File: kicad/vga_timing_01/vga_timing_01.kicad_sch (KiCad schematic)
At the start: 13 parts, among them J1 DIN41612_02x32_AC, J2 UART1, J3 UART2, U10 TL28L92FR, U13 74AHC1G32, Y1 Crystal 3.6864MHz

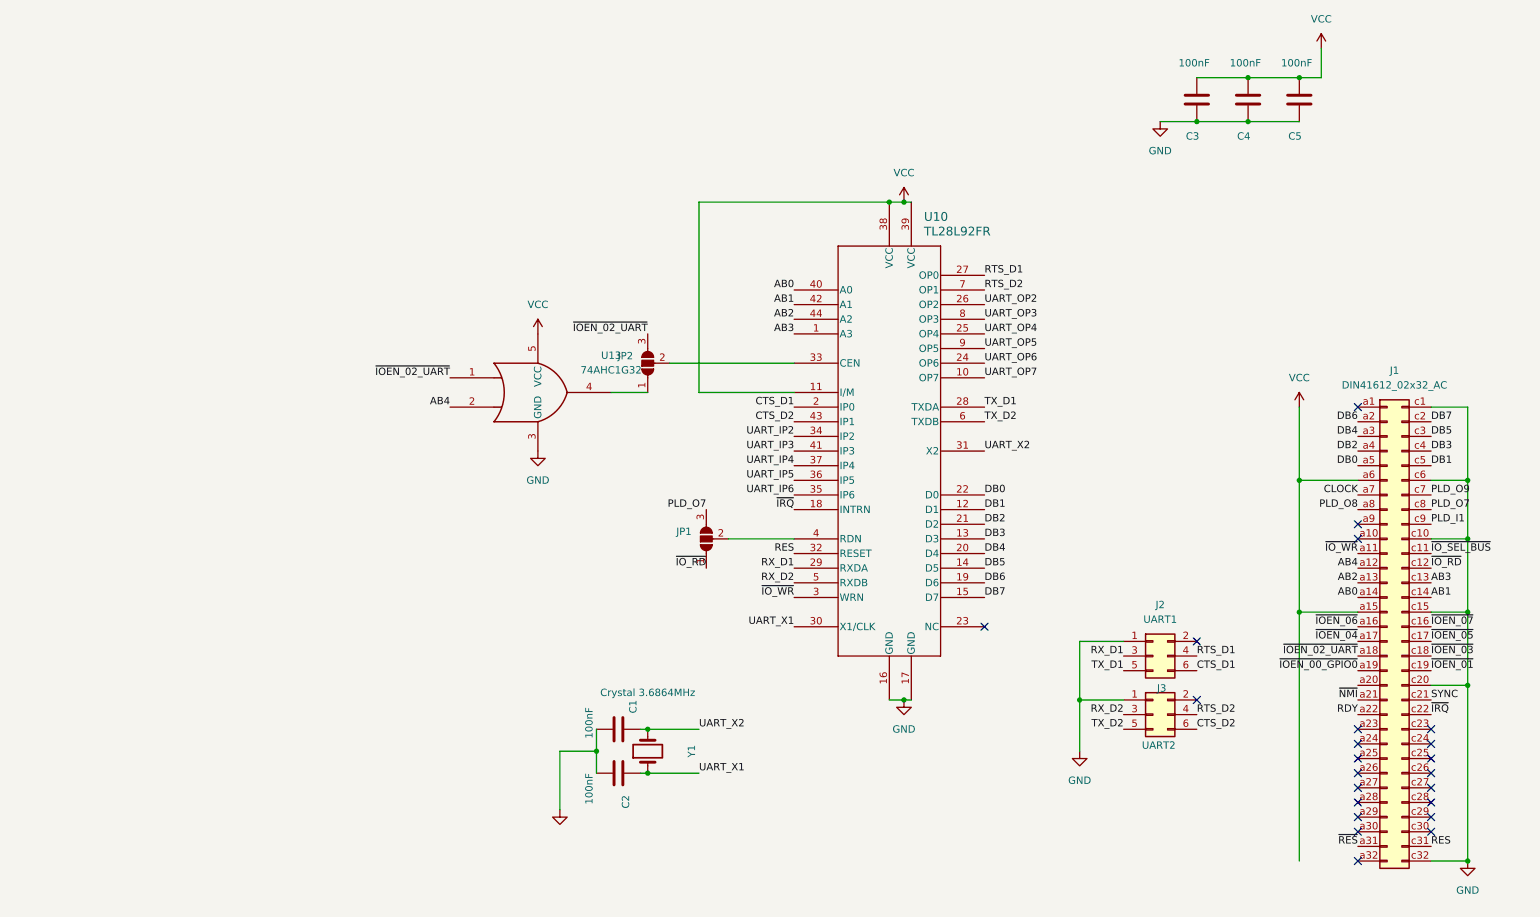
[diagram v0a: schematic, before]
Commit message: vga timing board 01 work
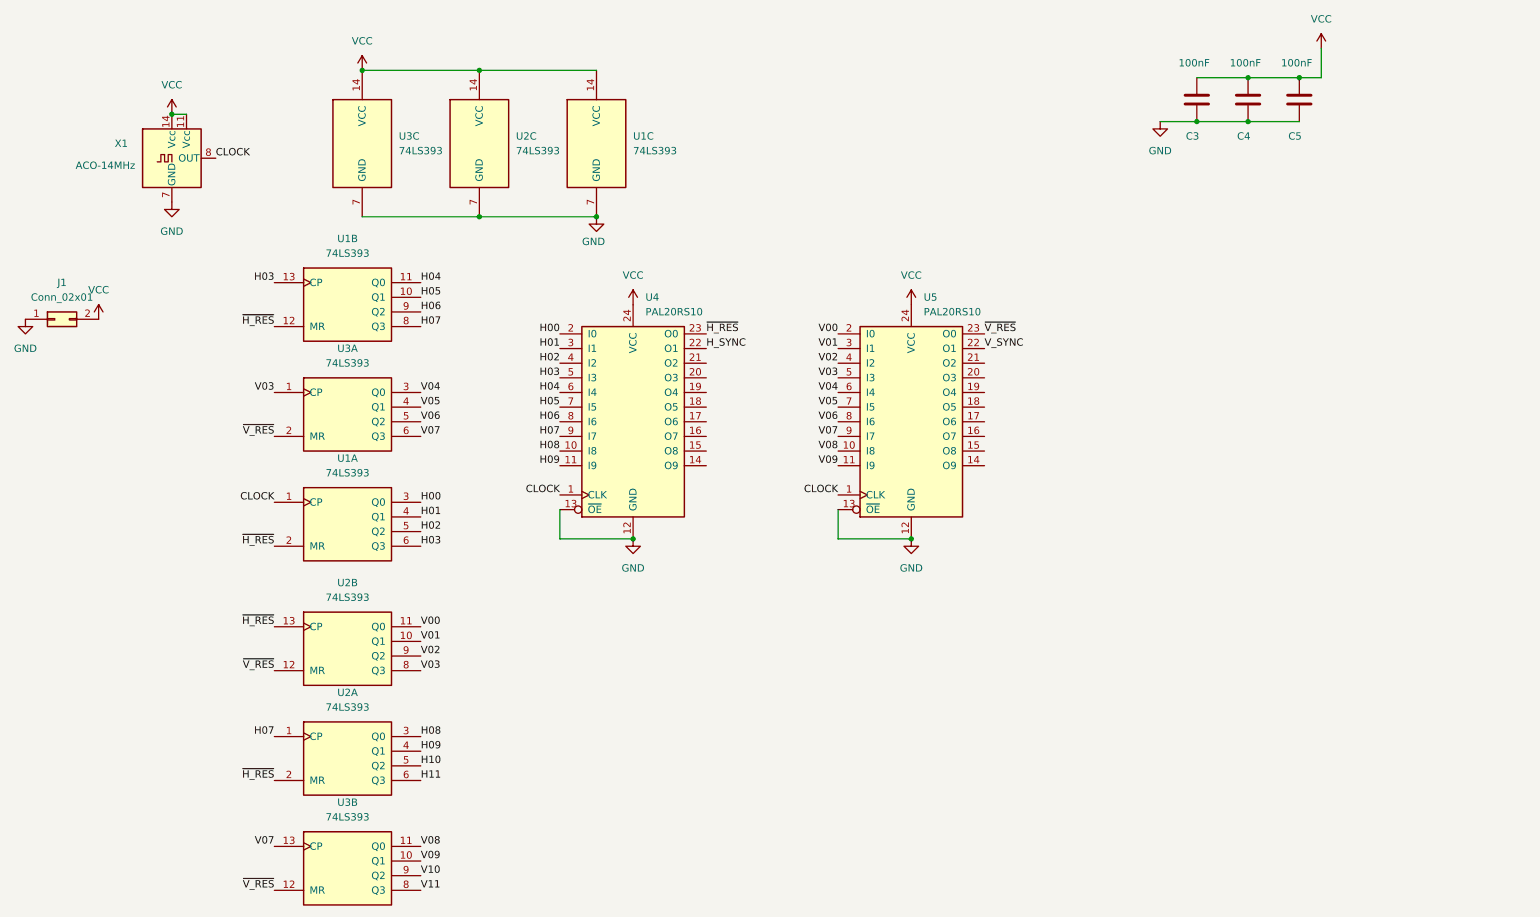
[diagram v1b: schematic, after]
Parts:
- removed C1, C2: 100nF, Capacitor_THT:C_Disc_D4.7mm_W2.5mm_P5.00mm, symbol Device:C
- removed J1: DIN41612_02x32_AC, Connector_DIN:DIN41612_C_2x32_Male_Horizontal_THT, symbol Connector:DIN41612_02x32_AC
- removed J2: UART1, Connector_PinHeader_2.54mm:PinHeader_2x03_P2.54mm_Horizontal, symbol Connector_Generic:Conn_02x03_Odd_Even
- removed J3: UART2, Connector_PinHeader_2.54mm:PinHeader_2x03_P2.54mm_Horizontal, symbol Connector_Generic:Conn_02x03_Odd_Even
- removed JP1, JP2: SolderJumper_3_Open, Jumper:SolderJumper-3_P1.3mm_Open_RoundedPad1.0x1.5mm_NumberLabels, symbol Jumper:SolderJumper_3_Open
- removed U10: TL28L92FR, Package_QFP:MQFP-44_10x10mm_P0.8mm, symbol 2024-09-25_17-04-06:TL28L92FR
- removed U13: 74AHC1G32, Package_TO_SOT_SMD:SOT-23-5_HandSoldering, symbol 74xGxx:74AHC1G32
- removed Y1: Crystal 3.6864MHz, Crystal:Crystal_HC49-4H_Vertical, symbol Device:Crystal
- added J1: Conn_02x01, Connector_PinSocket_1.27mm:PinSocket_2x01_P1.27mm_Vertical, symbol Connector_Generic:Conn_02x01
- added U1, U2, U3: 74LS393, Package_SO:SOIC-14_3.9x8.7mm_P1.27mm, symbol 74xx:74LS393
- added U4, U5: PAL20RS10, Package_DIP:DIP-24_W7.62mm_Socket, symbol Logic_Programmable:PAL20RS10
- added X1: ACO-14MHz, Package_DIP:DIP-14_W7.62mm_Socket, symbol 65xx:osci-14or8
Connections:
- net CLOCK: now also U1.1 (CP), U4.1 (CLK), U5.1 (CLK), X1.8 (OUT)
- net GND: now also J1.1 (Pin_1), U1.7 (GND), U2.7 (GND), U3.7 (GND), U4.12 (GND), U4.13 (~{OE}), U5.12 (GND), U5.13 (~{OE}), X1.7 (GND)
- net VCC: now also J1.2 (Pin_2), U1.14 (VCC), U2.14 (VCC), U3.14 (VCC), U4.24 (VCC), U5.24 (VCC), X1.11 (Vcc), X1.14 (Vcc)
- new net H00: U1.3 (Q0), U4.2 (I0)
- new net H01: U1.4 (Q1), U4.3 (I1)
- new net H02: U1.5 (Q2), U4.4 (I2)
- new net H03: U1.13 (CP), U1.6 (Q3), U4.5 (I3)
- new net H04: U1.11 (Q0), U4.6 (I4)
- new net H05: U1.10 (Q1), U4.7 (I5)
- new net H06: U1.9 (Q2), U4.8 (I6)
- new net H07: U1.8 (Q3), U2.1 (CP), U4.9 (I7)
- new net H08: U2.3 (Q0), U4.10 (I8)
- new net H09: U2.4 (Q1), U4.11 (I9)
- new net H10: U2.5 (Q2)
- new net H11: U2.6 (Q3)
- new net H_SYNC: U4.22 (O1)
- new net V00: U2.11 (Q0), U5.2 (I0)
- new net V01: U2.10 (Q1), U5.3 (I1)
- new net V02: U2.9 (Q2), U5.4 (I2)
- new net V03: U2.8 (Q3), U3.1 (CP), U5.5 (I3)
- new net V04: U3.3 (Q0), U5.6 (I4)
- new net V05: U3.4 (Q1), U5.7 (I5)
- new net V06: U3.5 (Q2), U5.8 (I6)
- new net V07: U3.13 (CP), U3.6 (Q3), U5.9 (I7)
- new net V08: U3.11 (Q0), U5.10 (I8)
- new net V09: U3.10 (Q1), U5.11 (I9)
- new net V10: U3.9 (Q2)
- new net V11: U3.8 (Q3)
- new net V_SYNC: U5.22 (O1)
- new net ~{H_RES}: U1.12 (MR), U1.2 (MR), U2.13 (CP), U2.2 (MR), U4.23 (O0)
- new net ~{V_RES}: U2.12 (MR), U3.12 (MR), U3.2 (MR), U5.23 (O0)
- no-connect marks 23 -> 0

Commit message: test kicad busses
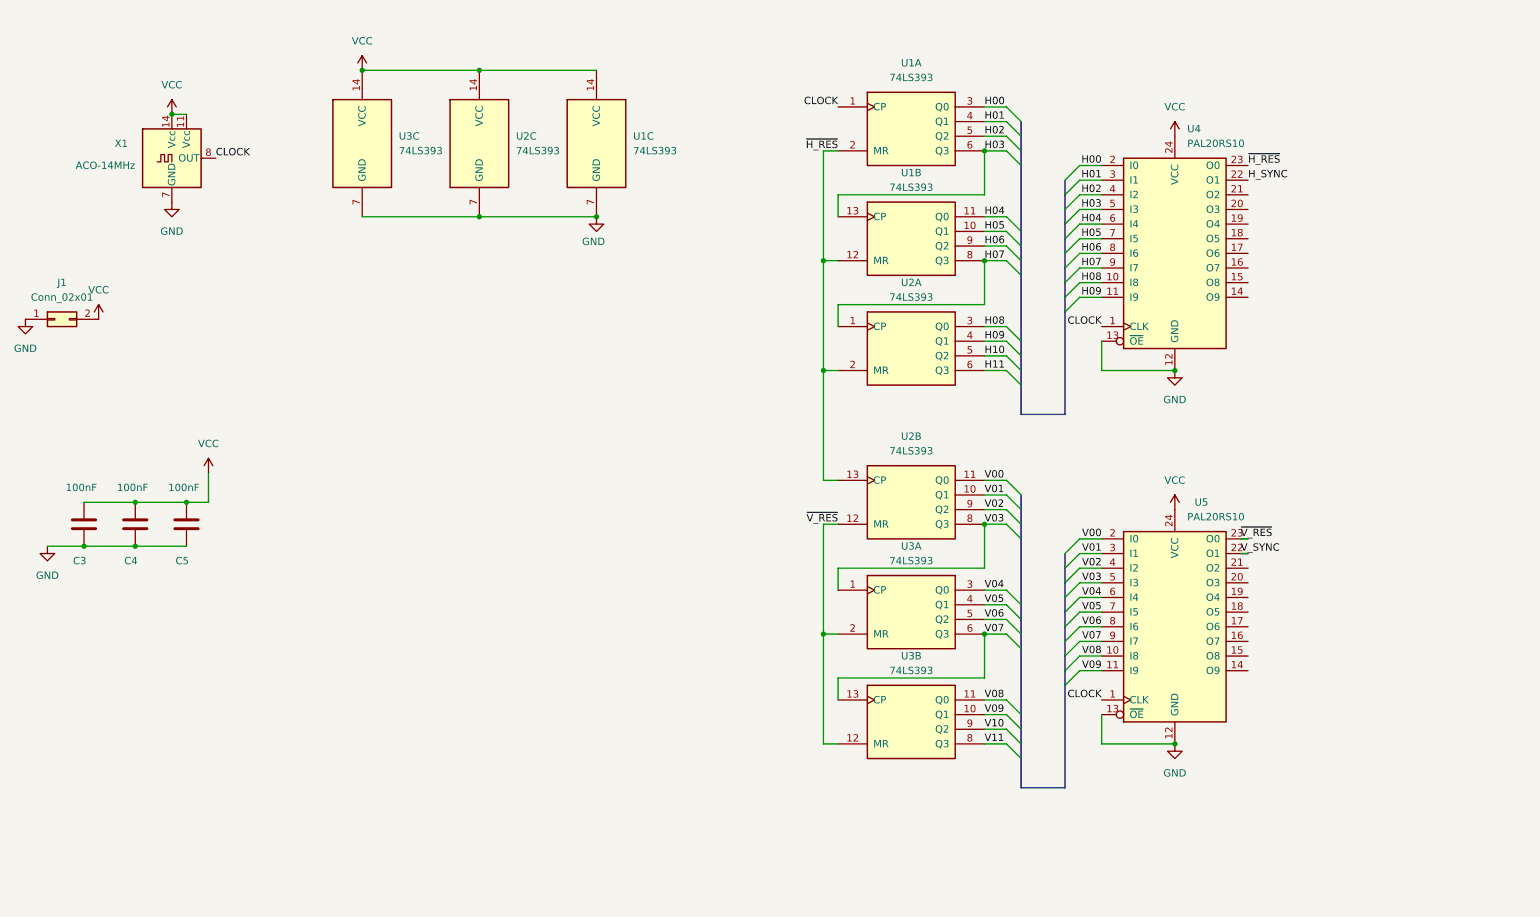
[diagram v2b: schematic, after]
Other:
- moved on the sheet: C3, C4, C5, U1A, U1B, U2A, U2B, U3A, U3B, U4, U5

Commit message: routing improvements
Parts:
- U1, U2, U3: footprint Package_SO:SOIC-14_3.9x8.7mm_P1.27mm -> Package_SO:SO-14_3.9x8.65mm_P1.27mm
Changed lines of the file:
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@@
 			)
 		)
-		(property "Footprint" "Package_SO:SOIC-14_3.9x8.7mm_P1.27mm"
+		(property "Footprint" "Package_SO:SO-14_3.9x8.65mm_P1.27mm"
 			(at 106.68 33.02 0)
 			(effects
@@
 			)
 		)
-		(property "Footprint" "Package_SO:SOIC-14_3.9x8.7mm_P1.27mm"
+		(property "Footprint" "Package_SO:SO-14_3.9x8.65mm_P1.27mm"
 			(at 181.61 67.31 0)
 			(effects
@@
 			)
 		)
-		(property "Footprint" "Package_SO:SOIC-14_3.9x8.7mm_P1.27mm"
+		(property "Footprint" "Package_SO:SO-14_3.9x8.65mm_P1.27mm"
 			(at 181.61 113.03 0)
 			(effects
@@
 			)
 		)
-		(property "Footprint" "Package_SO:SOIC-14_3.9x8.7mm_P1.27mm"
+		(property "Footprint" "Package_SO:SO-14_3.9x8.65mm_P1.27mm"
 			(at 181.61 29.21 0)
 			(effects
@@
 			)
 		)
-		(property "Footprint" "Package_SO:SOIC-14_3.9x8.7mm_P1.27mm"
+		(property "Footprint" "Package_SO:SO-14_3.9x8.65mm_P1.27mm"
 			(at 86.36 33.02 0)
 			(effects
@@
 			)
 		)
-		(property "Footprint" "Package_SO:SOIC-14_3.9x8.7mm_P1.27mm"
+		(property "Footprint" "Package_SO:SO-14_3.9x8.65mm_P1.27mm"
 			(at 181.61 93.98 0)
 			(effects
@@
 			)
 		)
-		(property "Footprint" "Package_SO:SOIC-14_3.9x8.7mm_P1.27mm"
+		(property "Footprint" "Package_SO:SO-14_3.9x8.65mm_P1.27mm"
 			(at 181.61 132.08 0)
 			(effects
@@
 			)
 		)
-		(property "Footprint" "Package_SO:SOIC-14_3.9x8.7mm_P1.27mm"
+		(property "Footprint" "Package_SO:SO-14_3.9x8.65mm_P1.27mm"
 			(at 127 33.02 0)
 			(effects
@@
 			)
 		)
-		(property "Footprint" "Package_SO:SOIC-14_3.9x8.7mm_P1.27mm"
+		(property "Footprint" "Package_SO:SO-14_3.9x8.65mm_P1.27mm"
 			(at 181.61 48.26 0)
 			(effects
